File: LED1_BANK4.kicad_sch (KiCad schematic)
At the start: 76 parts, among them U18 STP16CPC26T

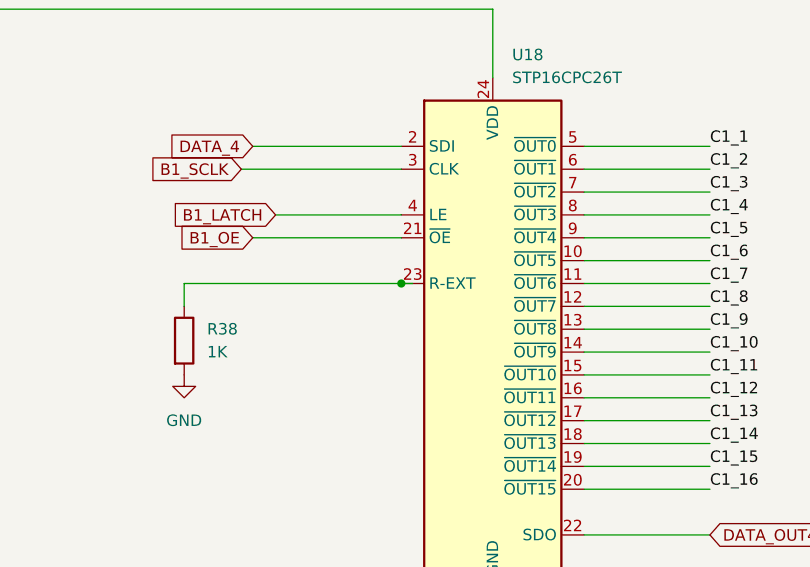
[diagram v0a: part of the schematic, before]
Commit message: sample
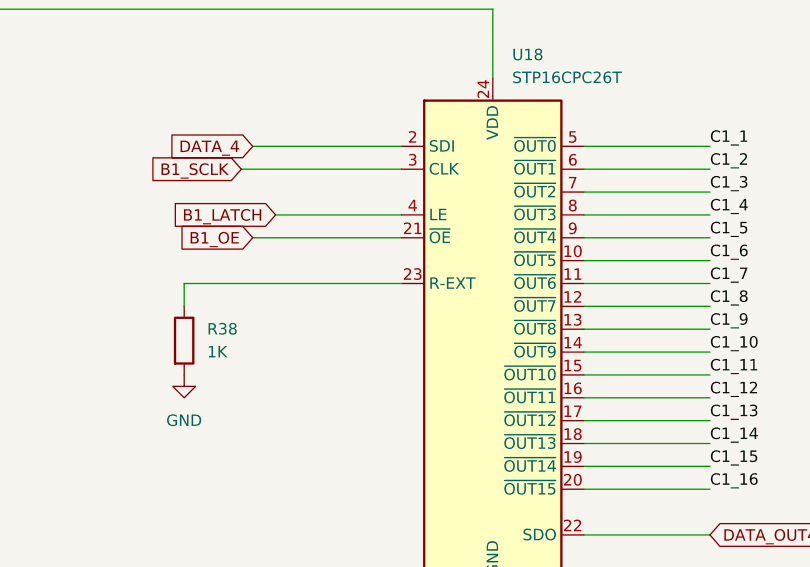
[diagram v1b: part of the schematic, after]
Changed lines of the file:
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@@
-	)
-	(junction
-		(at 82.55 160.02)
-		(diameter 0)
-		(color 0 0 0 0)
 	)
 	(junction
@@
 		)
 		(stroke
-			(width 0)
-			(type default)
-		)
-	)
-	(wire
-		(pts
-			(xy 82.55 160.02) (xy 83.82 160.02)
-		)
-		(stroke
